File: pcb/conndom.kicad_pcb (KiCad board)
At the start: 2 copper layers, 82 x 32 mm, 18 parts, among them J1 USB C PWR, J2 USB A WIFI

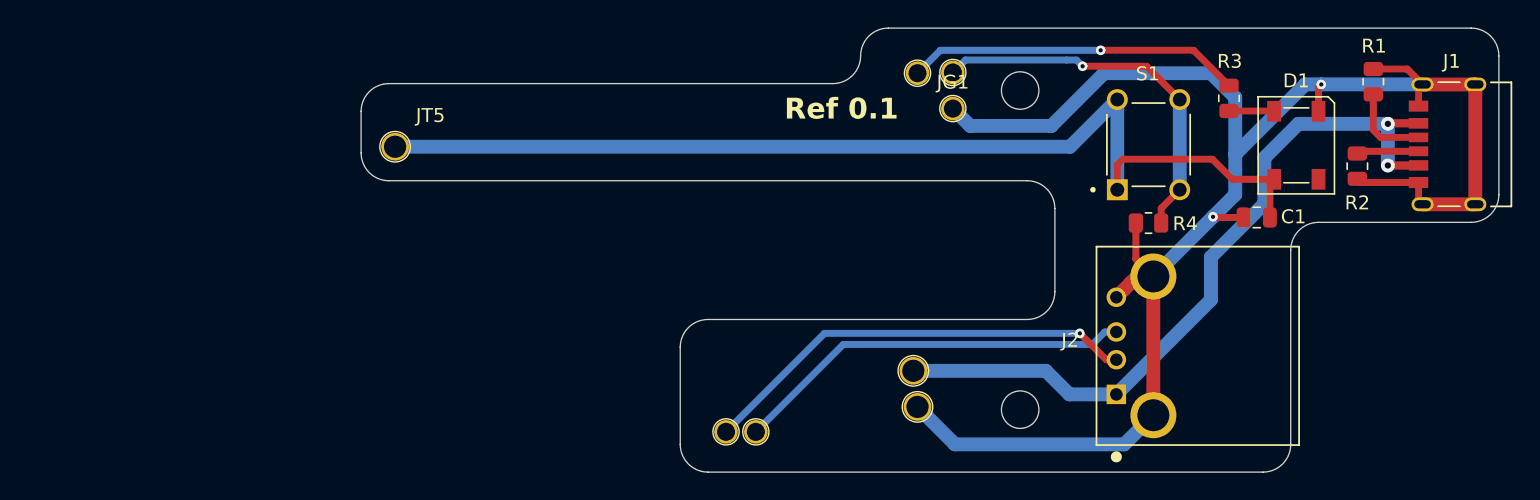
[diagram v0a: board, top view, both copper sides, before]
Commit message: pcb rev 0.2
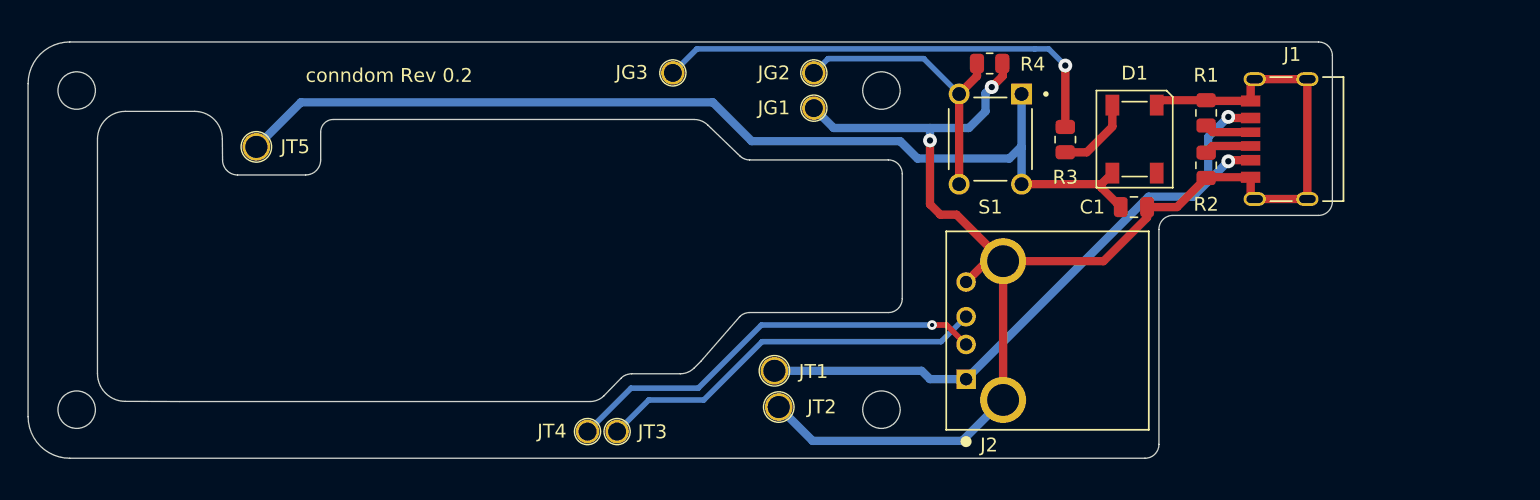
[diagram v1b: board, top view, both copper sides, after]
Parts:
- moved JG3 17.6 mm to (138.5, 82.2)
- moved R4 16.2 mm to (161.3, 81.5), turned to 180 degrees
- moved R1 12.3 mm to (176.9, 85.1)
- moved R3 12.2 mm to (166.8, 87.0)
- moved J1 12.1 mm to (184.2, 87.0)
- moved D1 11.7 mm to (171.7, 87.0)
- moved S1 11.4 mm to (161.3, 87.0), turned to -90 degrees
- moved R2 10.9 mm to (176.9, 88.9)
- moved J2 10.9 mm to (159.6, 104.3)
- moved JG1 10.0 mm to (148.6, 84.8)
- moved JG2 10.0 mm to (148.6, 82.2)
- moved JT1 10.0 mm to (145.8, 103.7)
- moved JT3 10.0 mm to (134.4, 108.1)
- moved JT2 10.0 mm to (146.1, 106.3)
- moved JT5 10.0 mm to (108.5, 87.6)
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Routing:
- net GND: track 123.7 -> 108.9 mm
- net Net-(JG3-Pin_1): track 24.2 -> 34.0 mm
- net Net-(JG2-Pin_1): track 27.4 -> 21.2 mm, vias 1 -> 0
- net +5V: track 54.2 -> 48.0 mm
- net Net-(J1-CC2): track 6.05 -> 3.41 mm
- net Net-(D1-VDD): track 76.7 -> 74.1 mm
- net Net-(D1-DIN): track 3.26 -> 5.71 mm
- net Net-(J1-CC1): track 4.48 -> 3.41 mm
- net Net-(JT4-Pin_1): track 31.9 -> 31.0 mm
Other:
- board size 82 x 32 mm -> 91 x 30 mm
- board text added: "conndom Rev 0.2"
- board text removed: "Ref 0.1"
